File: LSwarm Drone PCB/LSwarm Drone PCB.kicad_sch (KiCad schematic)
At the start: 128 parts, among them J1 Conn_01x04_Pin, J2 USB_C_Receptacle_USB2.0_16P, J3 JST / BT2.0 Connector, J4 Conn_01x02_Pin, J5 Conn_01x02_Pin, J6 Conn_01x02_Pin, J7 Conn_01x02_Pin, Q1 AO3400A, Q2 AO3400A, Q3 AO3400A, Q4 AO3400A, Q7 AO3407A, SW1 MSK12C02, U1 RP2350A, U10 LSM6DSR, U11 BMP581, U12 AP2112K-3.3, U13 TPS61023DRLR, U14 SN74LVC1T45DBVR, U4 W25Q128JVS, U6 ESP32-C3, Y1 12MHz, Y3 40MHz

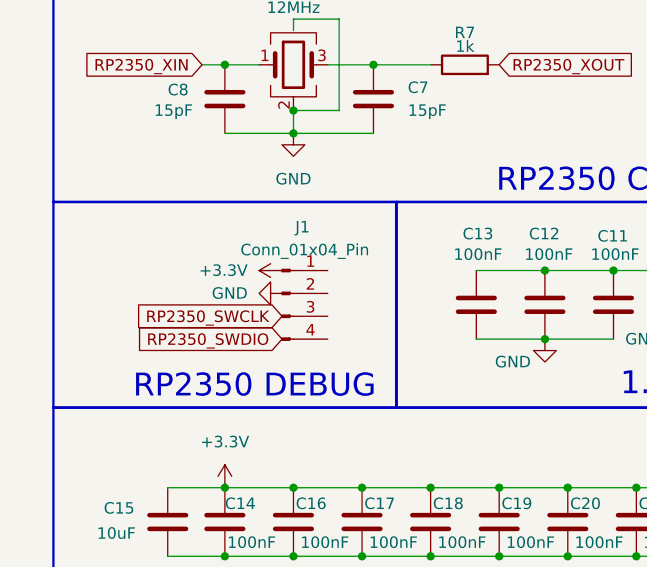
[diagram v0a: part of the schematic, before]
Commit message: finished pcb layout
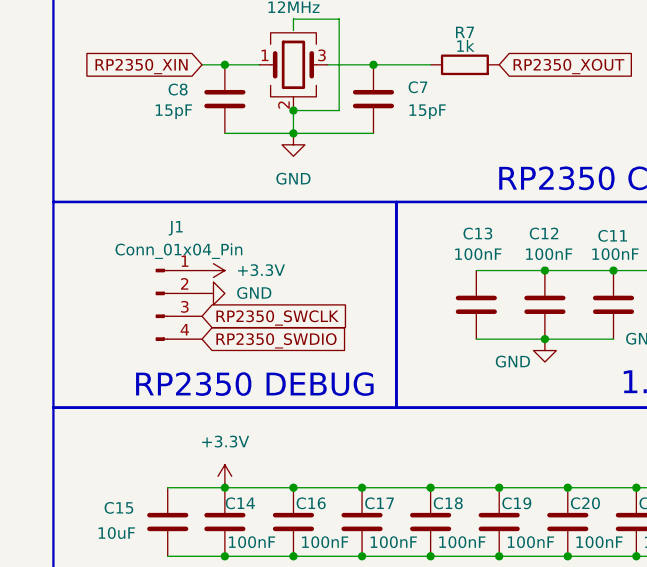
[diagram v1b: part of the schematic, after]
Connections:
- net +3.3V: now also J1.1 (Pin_1)
- net GND: now also J1.2 (Pin_2)
- net RP2350_SWCLK: now also J1.3 (Pin_3)
- net RP2350_SWDIO: now also J1.4 (Pin_4)
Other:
- moved on the sheet: J1
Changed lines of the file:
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@@
 	(global_label "RP2350_SWDIO"
 		(shape input)
-		(at 38.1 167.64 180)
+		(at 29.21 167.64 0)
 		(fields_autoplaced yes)
 		(effects
@@
 				(size 1.27 1.27)
 			)
-			(justify right)
+			(justify left)
 		)
 		(property "Intersheetrefs" "${INTERSHEET_REFS}"
-			(at 20.903 167.64 0)
+			(at 46.407 167.64 0)
 			(hide yes)
 			(show_name no)
@@
 					(size 1.27 1.27)
 				)
-				(justify right)
+				(justify left)
 			)
 		)
@@
 	(global_label "RP2350_SWCLK"
 		(shape input)
-		(at 38.1 165.1 180)
+		(at 29.21 165.1 0)
 		(fields_autoplaced yes)
 		(effects
@@
 				(size 1.27 1.27)
 			)
-			(justify right)
+			(justify left)
 		)
 		(property "Intersheetrefs" "${INTERSHEET_REFS}"
-			(at 20.5402 165.1 0)
+			(at 46.7698 165.1 0)
 			(hide yes)
 			(show_name no)
@@
 					(size 1.27 1.27)
 				)
-				(justify right)
+				(justify left)
 			)
 		)
@@
 	(symbol
 		(lib_id "power:+3.3V")
-		(at 38.1 160.02 90)
+		(at 29.21 160.02 270)
 		(unit 1)
 		(body_style 1)
@@
 		(fields_autoplaced yes)
 		(property "Reference" "#PWR038"
-			(at 41.91 160.02 0)
+			(at 25.4 160.02 0)
 			(hide yes)
 			(show_name no)
@@
 		)
 		(property "Value" "+3.3V"
-			(at 34.29 160.0199 90)
+			(at 33.02 160.0199 90)
 			(show_name no)
 			(do_not_autoplace no)
@@
 		)
 		(property "Footprint" ""
-			(at 38.1 160.02 0)
+			(at 29.21 160.02 0)
 			(hide yes)
 			(show_name no)
@@
 		)
 		(property "Datasheet" ""
-			(at 38.1 160.02 0)
+			(at 29.21 160.02 0)
 			(hide yes)
 			(show_name no)
@@
 		)
 		(property "Description" "Power symbol creates a global label with name \"+3.3V\""
-			(at 38.1 160.02 0)
+			(at 29.21 160.02 0)
 			(hide yes)
 			(show_name no)
@@
 	(symbol
 		(lib_id "Connector:Conn_01x04_Pin")
-		(at 38.1 162.56 0)
+		(at 24.13 162.56 0)
 		(unit 1)
 		(body_style 1)
@@
 		(dnp no)
 		(property "Reference" "J1"
-			(at 40.386 155.194 0)
+			(at 26.416 155.194 0)
 			(show_name no)
 			(do_not_autoplace no)
@@
 		)
 		(property "Value" "Conn_01x04_Pin"
-			(at 40.64 157.734 0)
+			(at 26.67 157.734 0)
 			(show_name no)
 			(do_not_autoplace no)
@@
 		)
 		(property "Footprint" "Connector_PinHeader_2.54mm:PinHeader_1x04_P2.54mm_Vertical"
-			(at 38.1 162.56 0)
+			(at 24.13 162.56 0)
 			(hide yes)
 			(show_name no)
@@
 		)
 		(property "Datasheet" ""
-			(at 38.1 162.56 0)
+			(at 24.13 162.56 0)
 			(hide yes)
 			(show_name no)
@@
 		)
 		(property "Description" "Generic connector, single row, 01x04, script generated"
-			(at 38.1 162.56 0)
+			(at 24.13 162.56 0)
 			(hide yes)
 			(show_name no)
@@
 	(symbol
 		(lib_id "power:GND")
-		(at 38.1 162.56 270)
+		(at 29.21 162.56 90)
 		(unit 1)
 		(body_style 1)
@@
 		(fields_autoplaced yes)
 		(property "Reference" "#PWR039"
-			(at 31.75 162.56 0)
+			(at 35.56 162.56 0)
 			(hide yes)
 			(show_name no)
@@
 		)
 		(property "Value" "GND"
-			(at 34.29 162.5599 90)
+			(at 33.02 162.5599 90)
 			(show_name no)
 			(do_not_autoplace no)
@@
 		)
 		(property "Footprint" ""
-			(at 38.1 162.56 0)
+			(at 29.21 162.56 0)
 			(hide yes)
 			(show_name no)
@@
 		)
 		(property "Datasheet" ""
-			(at 38.1 162.56 0)
+			(at 29.21 162.56 0)
 			(hide yes)
 			(show_name no)
@@
 		)
 		(property "Description" "Power symbol creates a global label with name \"GND\" , ground"
-			(at 38.1 162.56 0)
+			(at 29.21 162.56 0)
 			(hide yes)
 			(show_name no)
